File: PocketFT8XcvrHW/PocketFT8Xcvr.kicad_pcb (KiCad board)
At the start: 4 copper layers, 100 x 69.9 mm, 60 parts, among them J1 HX8357D SPI, J2 CONN SMA JACK STR 50OHM EDGE 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, J3 B5B-XH-A_LF__SN_, J5 HX8357D 8-BIT, Q1 2N7002DW, U1 MCP3422A1T-E/SN, U2 Si4735-D60-GU, U3 SN74ACT244DWR, U4 SI5351C-B-GM, Y1 ASTX-H11-25.000MHZ-T

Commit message: Cleanup for V2.00 fab
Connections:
- net Net-(FL1-IN) renamed /RF
- net Net-(FL1-OUT) renamed /ANT

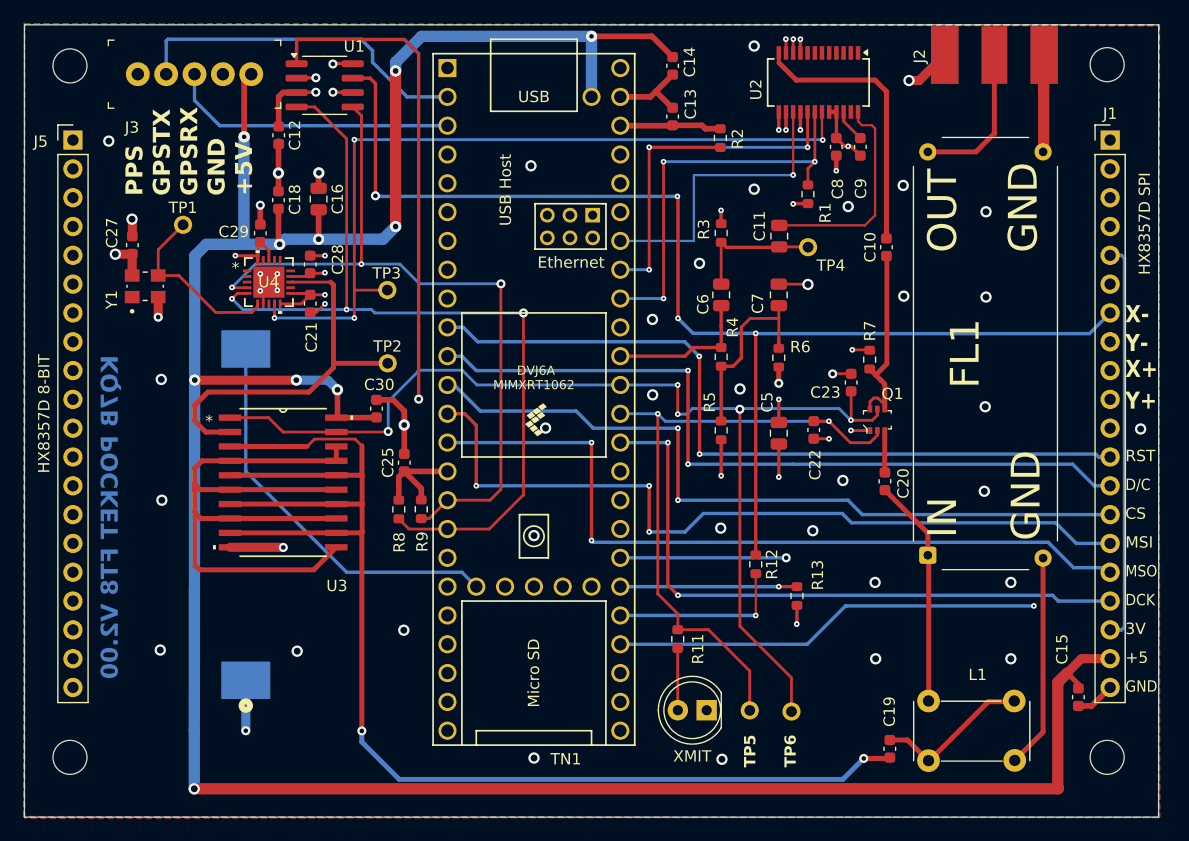
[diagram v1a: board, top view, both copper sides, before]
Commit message: V2.00 Submission to PCBWay
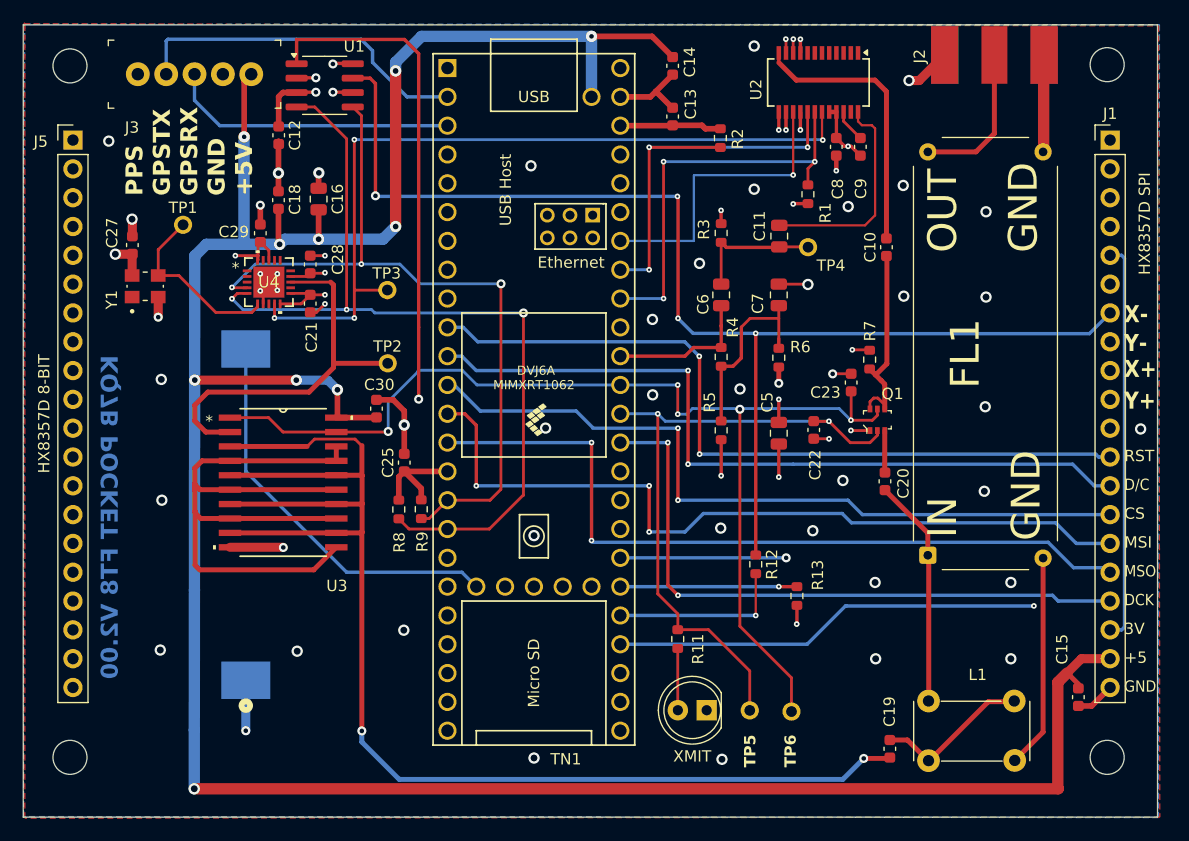
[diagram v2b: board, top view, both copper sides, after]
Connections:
- net Net-(U4-CLKIN) renamed /CLK
